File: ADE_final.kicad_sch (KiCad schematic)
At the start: 33 parts, among them J7 Conn_01x02_Pin, U10 ADE7953xCP, U8 ADE7953xCP, U9 MCP1825ST-3302E/EB, Y2 3.58M, Y3 3.58M

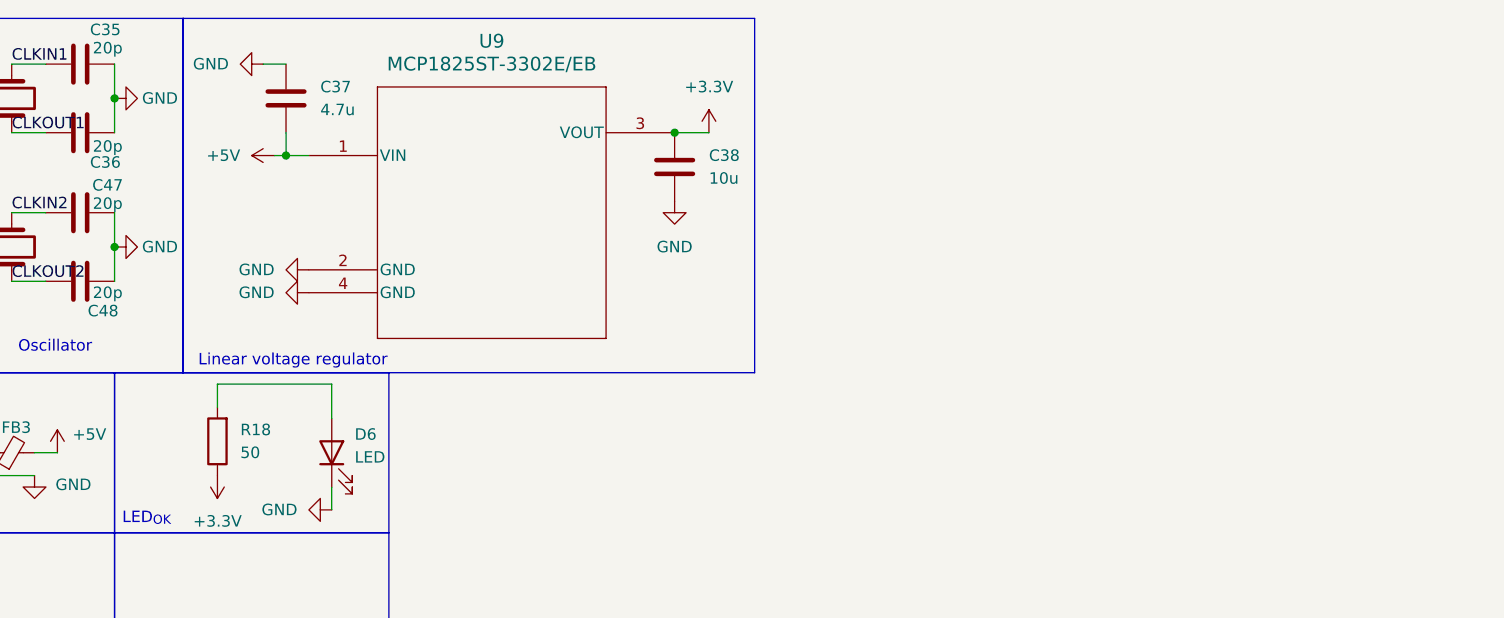
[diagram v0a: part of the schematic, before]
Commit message: NEW 1A LDO
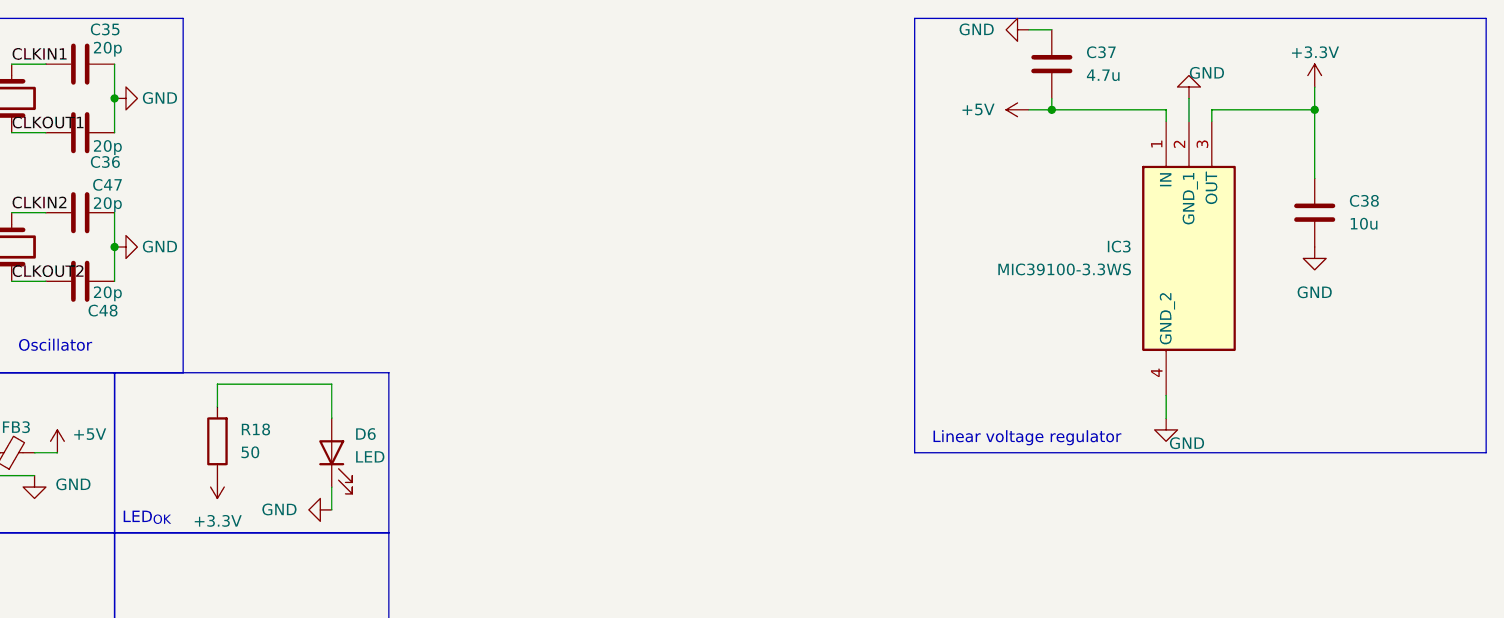
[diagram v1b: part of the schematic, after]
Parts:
- removed U9: MCP1825ST-3302E/EB, SmartSupplyLib:DDPAK3_MC_MCH, symbol SmartSupplyLib:MCP1825ST-3302E_EB
- added IC3: MIC39100-3.3WS, SOT230P700X180-4N, symbol SamacSys_Parts:MIC39100-3.3WS
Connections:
- net +3.3V: now also IC3.3 (OUT)
- net +5V: now also IC3.1 (IN)
- net GND: now also IC3.2 (GND_1), IC3.4 (GND_2)
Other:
- moved on the sheet: C37, C38
